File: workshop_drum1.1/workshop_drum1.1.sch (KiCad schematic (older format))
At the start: 32 parts, among them J1 9v_Battery_Clip, J2 Trigger_Input, J3 Output, U1 LM358, U2 7414, U3 78L05

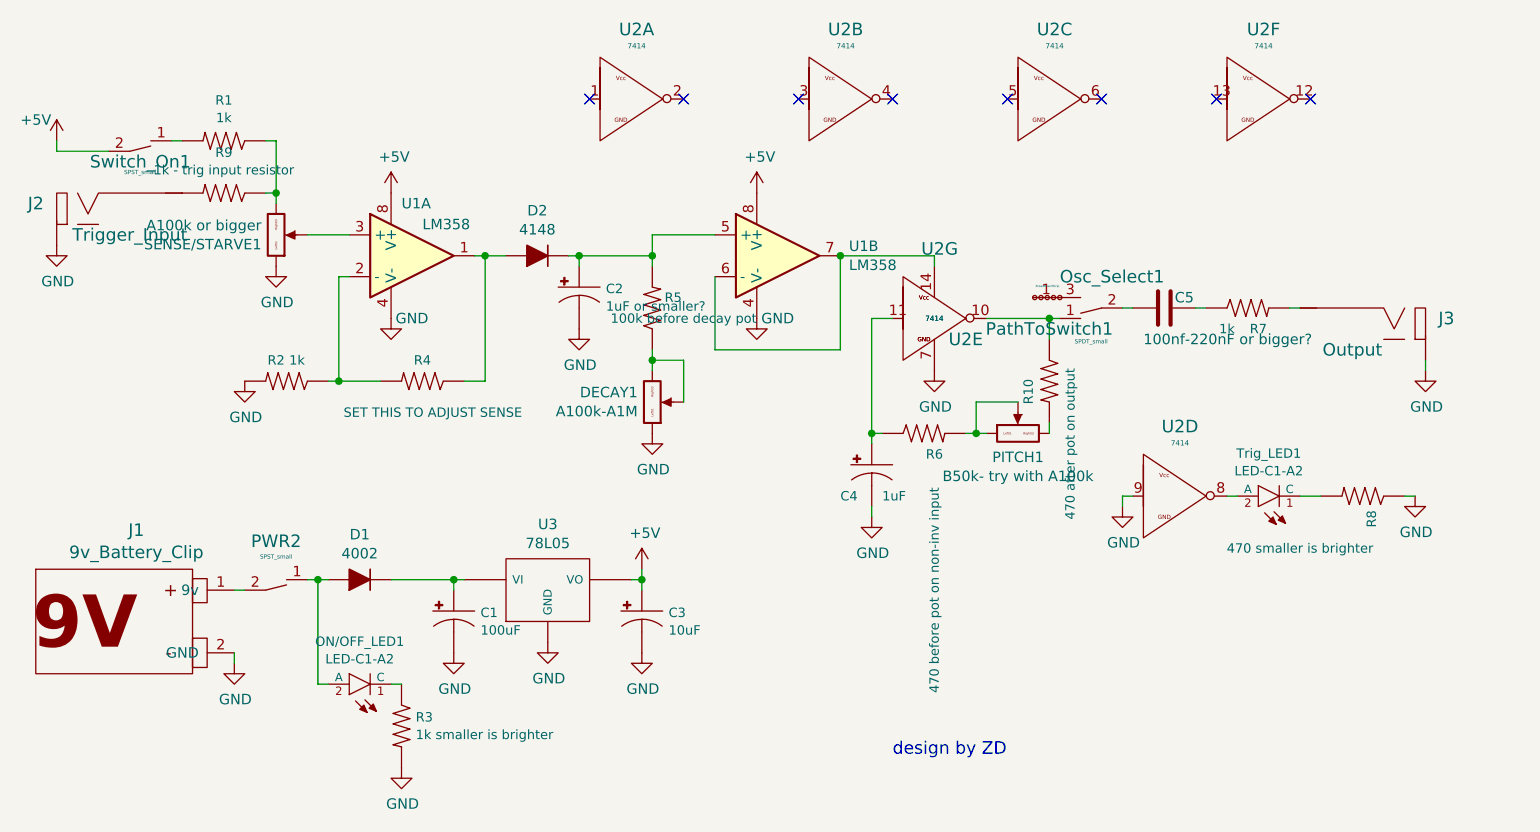
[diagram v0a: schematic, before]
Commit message: starting to lay traces
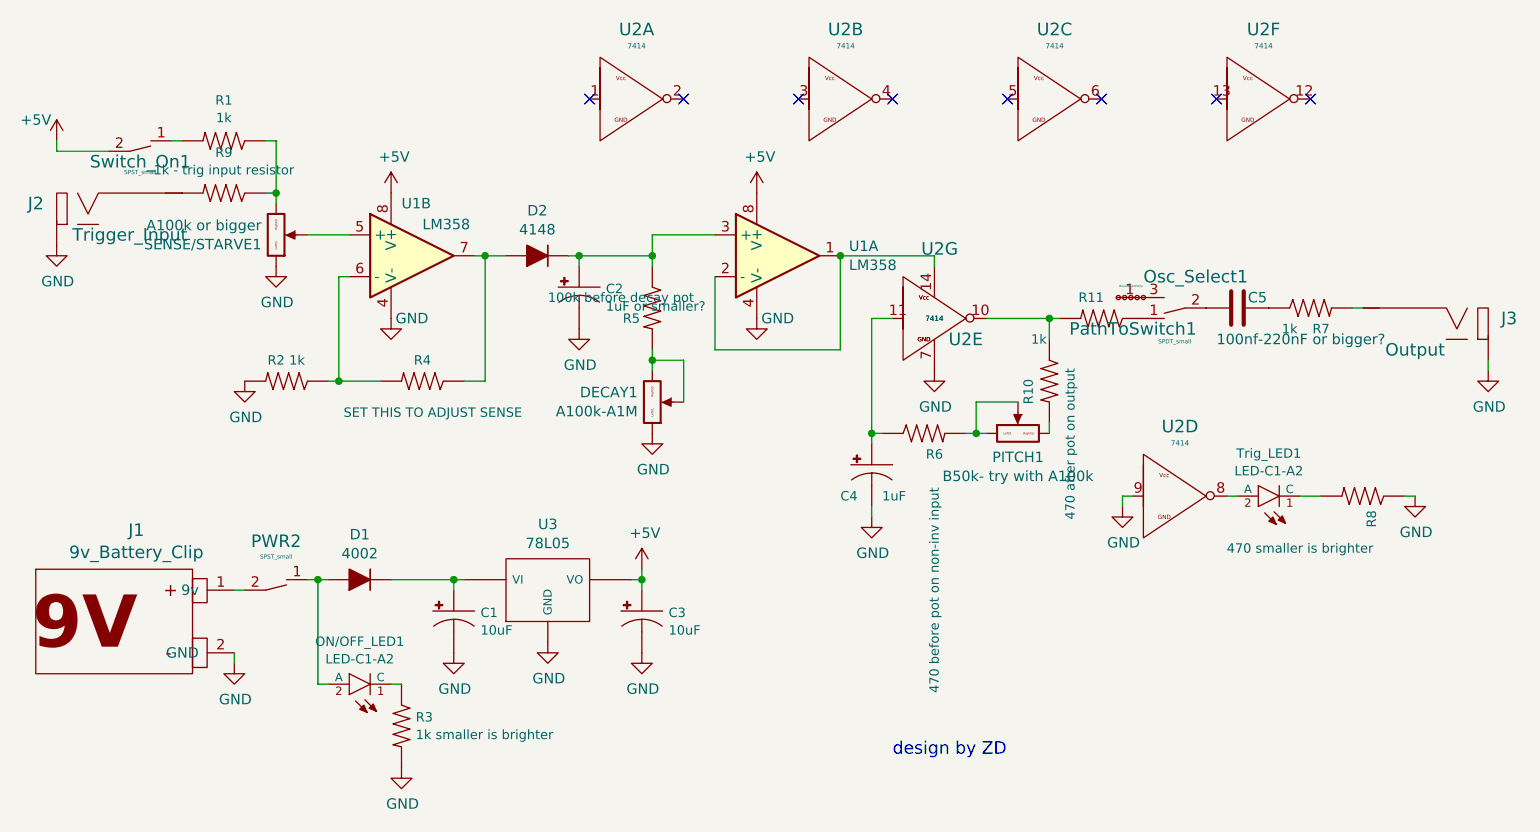
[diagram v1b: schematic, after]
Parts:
- added R11: 1k, 4ms-footprints:Resistor_TH_300, symbol 4ms-passives:RTH
- C1: value 100uF -> 10uF
- J1: footprint zfoot:Jack_DC -> zfoot:Jack_Instrument_Bigger
- J2, J3: footprint zfoot:Jack_Instrument -> zfoot:Jack_Instrument_Bigger
- U1: footprint 4ms-footprints:DIP_8pin_TL082_TH -> zfoot:DIP_8pin_TL082_TH_CenteredNotOnPin1
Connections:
- net at D2.2 (A), R4.1: now also U1.7; no longer U1.1
- net at R2.1, R4.2: now also U1.6 (-); no longer U1.2 (-)
- net at SENSE/STARVE1.2 (Center): now also U1.5 (+); no longer U1.3 (+)
- net at C2.1 (+), D2.1 (K): now also R5.1, U1.3 (+); no longer R5.2, U1.5 (+)
- net at R10.1, U2.10: now also R11.2; no longer Osc_Select1.1
- net at DECAY1.2 (Center), DECAY1.3 (Right): now also R5.2; no longer R5.1
- new net: U1.1, U1.2 (-), U2.14
- new net: Osc_Select1.1, R11.1
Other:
- moved on the sheet: C5, J3, Osc_Select1, PathToSwitch1, R7
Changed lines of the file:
@@
 $Comp
 L linear1:LM358 U1
-U 1 1 5A324A57
+U 2 1 5A324A57
 P 2450 1650
 F 0 "U1" H 2400 1900 50  0000 L CNN
 F 1 "LM358" H 2500 1800 50  0000 L CNN
-F 2 "4ms-footprints:DIP_8pin_TL082_TH" H 2450 1650 50  0001 C CNN
+F 2 "zfoot:DIP_8pin_TL082_TH_CenteredNotOnPin1" H 2450 1650 50  0001 C CNN
 F 3 "" H 2450 1650 50  0001 C CNN
-	1    2450 1650
+	2    2450 1650
 	1    0    0    -1
 $EndComp
 $Comp
 L linear1:LM358 U1
-U 2 1 5A324B18
+U 1 1 5A324B18
 P 4200 1650
 F 0 "U1" H 4541 1696 50  0000 L CNN
 F 1 "LM358" H 4541 1605 50  0000 L CNN
-F 2 "4ms-footprints:DIP_8pin_TL082_TH" H 4200 1650 50  0001 C CNN
+F 2 "zfoot:DIP_8pin_TL082_TH_CenteredNotOnPin1" H 4200 1650 50  0001 C CNN
 F 3 "" H 4200 1650 50  0001 C CNN
-	2    4200 1650
+	1    4200 1650
 	1    0    0    -1
 $EndComp
@@
 F 0 "J1" H 1131 3837 60  0000 C CNN
 F 1 "9v_Battery_Clip" H 1131 3731 60  0000 C CNN
-F 2 "zfoot:Jack_DC" H 1100 3400 60  0001 C CNN
+F 2 "zfoot:Jack_Instrument_Bigger" H 1100 3400 60  0001 C CNN
 F 3 "" H 1100 3400 60  0001 C CNN
 	1    1100 3400
@@
 P 2650 3350
 F 0 "C1" H 2778 3342 45  0000 L CNN
-F 1 "100uF" H 2778 3258 45  0000 L CNN
+F 1 "10uF" H 2778 3258 45  0000 L CNN
 F 2 "4ms-footprints:Cap_Electrolytic_TH" H 2680 3500 20  0001 C CNN
 F 3 "" H 2650 3350 60  0001 C CNN
@@
 L 4ms-passives:CAP_TH C5
 U 1 1 5A3339E6
-P 6050 1900
-F 0 "C5" V 6000 1950 50  0000 L CNN
-F 1 "100nf-220nF or bigger?" V 6200 1800 50  0000 L CNN
-F 2 "4ms-footprints:Cap_Ceramic_TH" H 6088 1750 50  0001 C CNN
-F 3 "" H 6050 1900 50  0001 C CNN
-	1    6050 1900
+P 6400 1900
+F 0 "C5" V 6350 1950 50  0000 L CNN
+F 1 "100nf-220nF or bigger?" V 6550 1800 50  0000 L CNN
+F 2 "4ms-footprints:Cap_Ceramic_TH" H 6438 1750 50  0001 C CNN
+F 3 "" H 6400 1900 50  0001 C CNN
+	1    6400 1900
 	0    1    1    0
 $EndComp
@@
 L zMECH:SPDT_small Osc_Select1
 U 1 1 5A3358B6
-P 5700 1900
-F 0 "Osc_Select1" H 5600 1750 60  0000 C CNN
-F 1 "SPDT_small" H 5700 2060 20  0000 C CNN
-F 2 "zfoot:Switch_Toggle_SPDT_Mini_SolderLug" H 5700 1900 60  0001 C CNN
-F 3 "" H 5700 1900 60  0001 C CNN
-	1    5700 1900
+P 6100 1900
+F 0 "Osc_Select1" H 6000 1750 60  0000 C CNN
+F 1 "SPDT_small" H 6100 2060 20  0000 C CNN
+F 2 "zfoot:Switch_Toggle_SPDT_Mini_SolderLug" H 6100 1900 60  0001 C CNN
+F 3 "" H 6100 1900 60  0001 C CNN
+	1    6100 1900
 	-1   0    0    1
 $EndComp
@@
 F 0 "J2" H 650 1600 60  0000 C CNN
 F 1 "Trigger_Input" H 1100 1450 60  0000 C CNN
-F 2 "zfoot:Jack_Instrument" H 900 1500 60  0001 C CNN
+F 2 "zfoot:Jack_Instrument_Bigger" H 900 1500 60  0001 C CNN
 F 3 "" H 900 1500 60  0000 C CNN
 	1    900  1500
@@
 F 3 "" H 3600 1900 60  0001 C CNN
 	1    3600 1900
-	0    -1   -1   0
+	0    1    1    0
 $EndComp
 $Comp
@@
 Wire Wire Line
 	5150 2350 5350 2350
-Wire Wire Line
-	5850 1900 5900 1900
 $Comp
 L 4ms-passives:RTH R7
 U 1 1 5A33161A
-P 6450 1900
-F 0 "R7" H 6500 1800 45  0000 C CNN
-F 1 "1k" H 6350 1800 45  0000 C CNN
-F 2 "4ms-footprints:Resistor_TH_300" H 6480 2050 20  0001 C CNN
-F 3 "" H 6450 1900 60  0001 C CNN
-	1    6450 1900
-	1    0    0    -1
-$EndComp
-Wire Wire Line
-	6200 1900 6250 1900
+P 6750 1900
+F 0 "R7" H 6800 1800 45  0000 C CNN
+F 1 "1k" H 6650 1800 45  0000 C CNN
+F 2 "4ms-footprints:Resistor_TH_300" H 6780 2050 20  0001 C CNN
+F 3 "" H 6750 1900 60  0001 C CNN
+	1    6750 1900
+	1    0    0    -1
+$EndComp
 $Comp
 L zMECH:JACK-TIP_GND J3
 U 1 1 5A331971
-P 7150 2050
-F 0 "J3" H 6900 2150 60  0000 C CNN
-F 1 "Output" H 7350 2000 60  0000 C CNN
-F 2 "zfoot:Jack_Instrument" H 7150 2050 60  0001 C CNN
-F 3 "" H 7150 2050 60  0000 C CNN
-	1    7150 2050
+P 7450 2050
+F 0 "J3" H 7200 2150 60  0000 C CNN
+F 1 "Output" H 7650 2000 60  0000 C CNN
+F 2 "zfoot:Jack_Instrument_Bigger" H 7450 2050 60  0001 C CNN
+F 3 "" H 7450 2050 60  0000 C CNN
+	1    7450 2050
 	-1   0    0    -1
 $EndComp
 Wire Wire Line
-	6650 1900 6700 1900
+	6950 1900 7000 1900
 $Comp
 L 4ms-power:GND #PWR018
 U 1 1 5A331D26
-P 7300 2200
-F 0 "#PWR018" H 7300 1950 50  0001 C CNN
-F 1 "GND" H 7305 2027 50  0000 C CNN
-F 2 "" H 7300 2200 50  0001 C CNN
-F 3 "" H 7300 2200 50  0001 C CNN
-	1    7300 2200
-	1    0    0    -1
-$EndComp
-Wire Wire Line
-	7300 2150 7300 2200
+P 7600 2200
+F 0 "#PWR018" H 7600 1950 50  0001 C CNN
+F 1 "GND" H 7605 2027 50  0000 C CNN
+F 2 "" H 7600 2200 50  0001 C CNN
+F 3 "" H 7600 2200 50  0001 C CNN
+	1    7600 2200
+	1    0    0    -1
+$EndComp
+Wire Wire Line
+	7600 2150 7600 2200
 $Comp
 L 4ms-power:GND #PWR019
@@
 L zMECH:BreadBoardStrip PathToSwitch1
 U 1 1 5A33DD61
-P 5550 1850
-F 0 "PathToSwitch1" H 5600 2000 60  0000 C CNN
-F 1 "BreadBoardStrip" H 5609 1795 10  0000 C CNN
-F 2 "zfoot:BREAKOUTswitch" H 5420 1830 60  0001 C CNN
-F 3 "" H 5550 1850 60  0001 C CNN
-	1    5550 1850
+P 5950 1850
+F 0 "PathToSwitch1" H 6000 2000 60  0000 C CNN
+F 1 "BreadBoardStrip" H 6009 1795 10  0000 C CNN
+F 2 "zfoot:BREAKOUTswitch" H 5820 1830 60  0001 C CNN
+F 3 "" H 5950 1850 60  0001 C CNN
+	1    5950 1850
 	-1   0    0    1
 $EndComp
@@
 Wire Wire Line
 	1800 1350 1800 1400
-Wire Wire Line
-	5200 1950 5500 1950
 $Comp
 L 4ms-passives:RTH R10
@@
 $EndComp
 Wire Wire Line
-	5500 1950 5500 2050
-Connection ~ 5500 1950
-Wire Wire Line
-	5500 1950 5550 1950
-Wire Wire Line
 	5500 2450 5500 2500
 Wire Wire Line
@@
 NoConn ~ 5300 900
 NoConn ~ 5750 900
+$Comp
+L 4ms-passives:RTH R11
+U 1 1 5AC19556
+P 5750 1950
+F 0 "R11" H 5800 1850 45  0000 C CNN
+F 1 "1k" H 6050 2050 45  0000 C CNN
+F 2 "4ms-footprints:Resistor_TH_300" H 5780 2100 20  0001 C CNN
+F 3 "" H 5750 1950 60  0001 C CNN
+	1    5750 1950
+	-1   0    0    1
+$EndComp
+Wire Wire Line
+	5550 1950 5500 1950
+Wire Wire Line
+	5500 2050 5500 1950
+Connection ~ 5500 1950
+Wire Wire Line
+	5500 1950 5200 1950
 $EndSCHEMATC

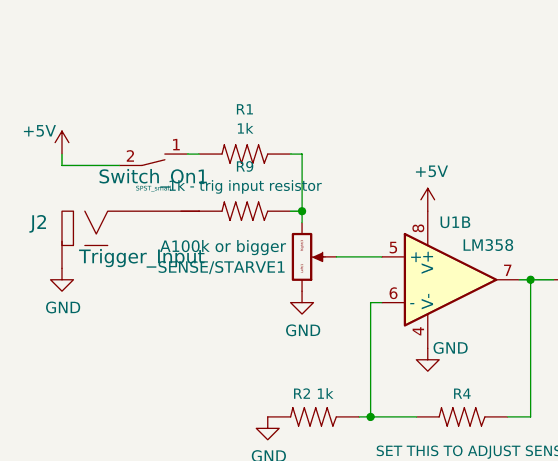
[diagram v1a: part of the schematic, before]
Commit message: Ready for review
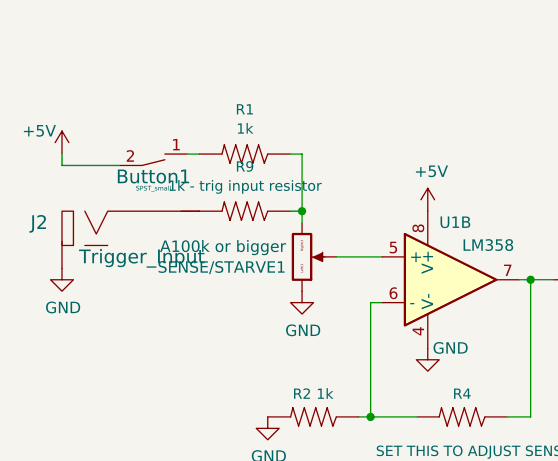
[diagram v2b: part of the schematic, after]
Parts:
- renumbered Switch_On1 to Button1
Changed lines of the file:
@@
 $EndComp
 $Comp
-L zMECH:SPST_small Switch_On1
+L zMECH:SPST_small Button1
 U 1 1 5A33654C
 P 1150 1150
-F 0 "Switch_On1" H 1150 1100 60  0000 C CNN
+F 0 "Button1" H 1150 1100 60  0000 C CNN
 F 1 "SPST_small" H 1150 1050 20  0000 C CNN
 F 2 "zfoot:Jack_Instrument_Bigger" H 1150 1150 60  0001 C CNN
